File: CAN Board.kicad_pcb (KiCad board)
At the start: 4 copper layers, 35 x 50 mm, 97 parts, among them J1 Conn_02x07_Odd_Even, J3 USB_C_Receptacle_USB2.0_16P, J4 Conn_01x02, J5 Conn_01x02, J6 Conn_01x02, J7 Conn_01x02, J8 Conn_01x02, J9 Conn_01x02, SW1 SW_Push, SW2 SW_Push, U1 RP2040, U2 W25Q128JVS, U3 MIC5504-3.3YM5, U4 MCP251863T-E/9PX, U5 MCP251863T-E/9PX, U6 MCP251863T-E/9PX, U7 MCP251863T-E/9PX, U8 MCP251863T-E/9PX, U9 MCP251863T-E/9PX, Y1 Crystal_GND24, Y2 Crystal_GND24, Y3 Crystal_GND24, Y4 Crystal_GND24, Y5 Crystal_GND24, Y6 Crystal_GND24, Y7 Crystal_GND24

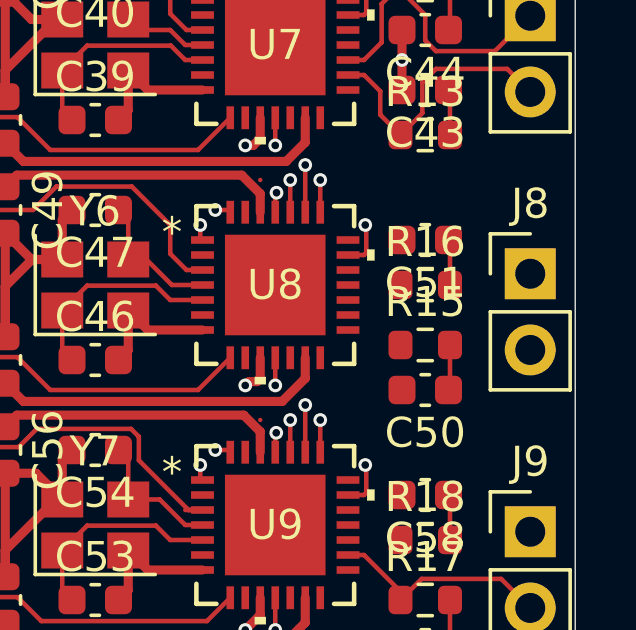
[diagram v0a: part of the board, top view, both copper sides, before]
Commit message: moving components
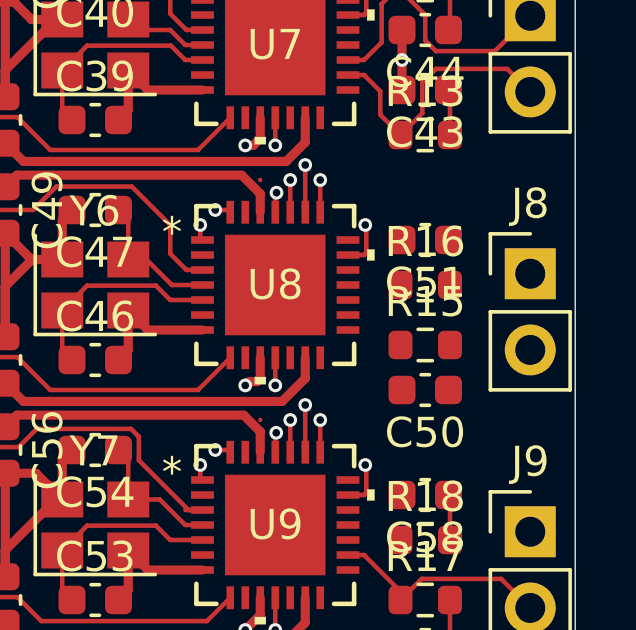
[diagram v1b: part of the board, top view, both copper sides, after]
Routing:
- net Net-(C51-Pad1): track 1.52 -> 0.07 mm
- net Net-(C50-Pad1): track 1.52 -> 0.07 mm
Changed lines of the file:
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@@
-	)
-	(segment
-		(start 57.825 51)
-		(end 57.825 52.45)
-		(width 0.1524)
-		(layer "F.Cu")
-		(net 18)
 	)
 	(segment
@@
 	)
 	(segment
-		(start 57.825 49)
-		(end 57.825 47.55)
-		(width 0.1524)
-		(layer "F.Cu")
-		(net 19)
-	)
-	(segment
